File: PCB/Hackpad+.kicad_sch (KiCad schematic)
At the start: 29 parts, among them SW1 RotaryEncoder_Switch, SW10 SW_Push, SW13 SW_Push, SW14 SW_Push, SW15 SW_Push, SW16 SW_Push, SW17 SW_Push, SW18 SW_Push, SW4 SW_Push, SW7 SW_Push, U1 XIAO-RP2040-DIP

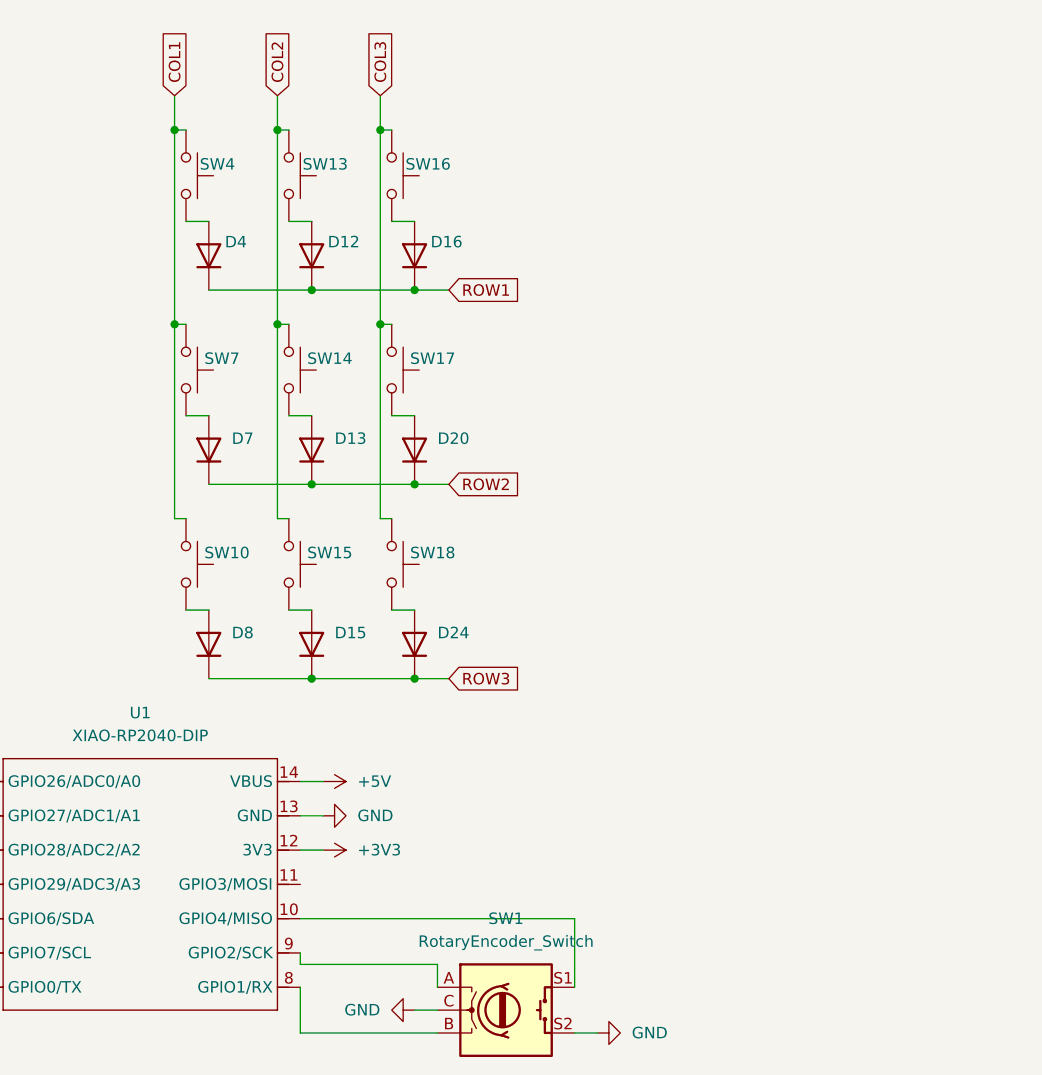
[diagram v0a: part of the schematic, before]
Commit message: changed files
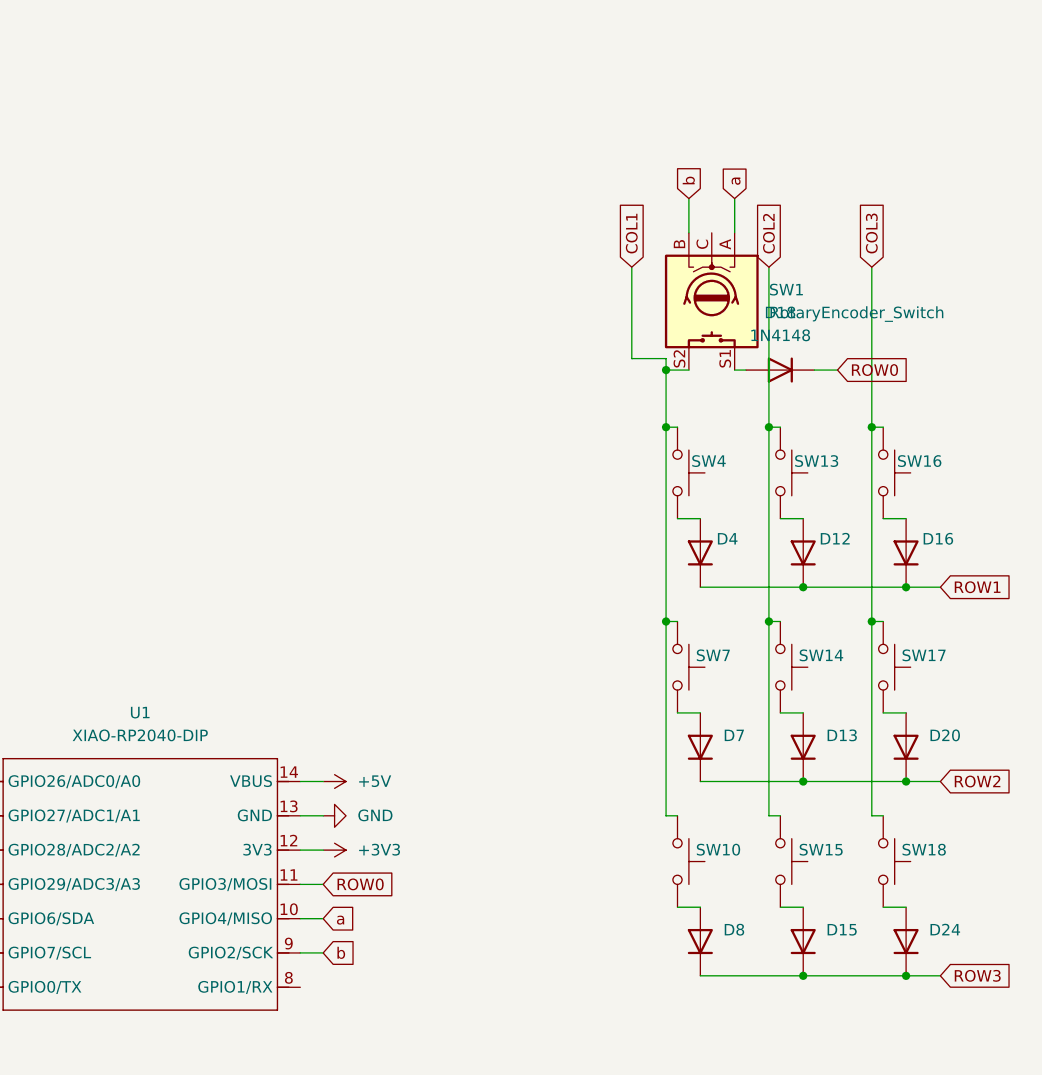
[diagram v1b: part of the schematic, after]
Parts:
- added D18: 1N4148, Diode_THT:D_DO-35_SOD27_P7.62mm_Horizontal, symbol Diode:1N4148
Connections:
- net COL1: now also SW1.S2
- net GND: no longer SW1.C, SW1.S2
- net at SW1.S1: now also D18.2 (A); no longer U1.10 (GPIO4/MISO)
- net ROW0: now reaches U1.11 (GPIO3/MOSI)
- net ROW0: now also D18.1 (K)
- net at U1.8 (GPIO1/RX): no longer SW1.B
- net a: now reaches SW1.A
- net a: now also U1.10 (GPIO4/MISO); no longer U1.9 (GPIO2/SCK)
- new net b: SW1.B, U1.9 (GPIO2/SCK)
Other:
- moved on the sheet: D12, D13, D15, D16, D20, D24, D4, D7, D8, SW1, SW10, SW13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
